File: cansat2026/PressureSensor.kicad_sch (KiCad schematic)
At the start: 2 parts, among them U601 AE-BME280

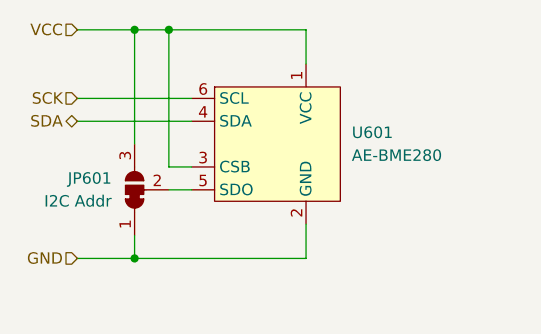
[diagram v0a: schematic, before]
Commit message: Update: いろいろした
無線変えた
カメラのコネクタ変えた
i2cセンサ変えた
電源変えた:1.2V,3.8V,3.3V
IOエキスパンダ追加
FPGA追加
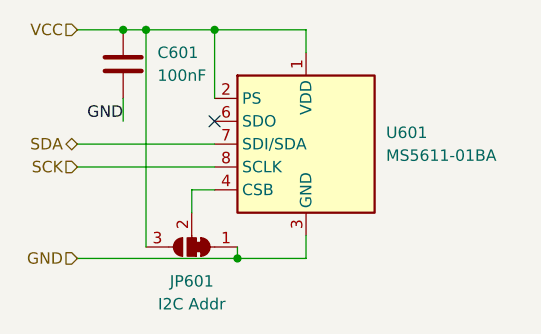
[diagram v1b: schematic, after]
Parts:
- removed U601: AE-BME280, Project:AE-BME280, symbol Project:AE-BME280
- added C601: 100nF, Capacitor_SMD:C_0402_1005Metric, symbol Device:C
- added U601: MS5611-01BA, Package_LGA:LGA-8_3x5mm_P1.25mm, symbol Sensor_Pressure:MS5611-01BA
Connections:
- net GND: now also C601.2, U601.3 (GND)
- net SCK: now also U601.8 (SCLK)
- net SDA: now also U601.7 (SDI/SDA)
- net VCC: now also C601.1, U601.1 (VDD), U601.2 (PS)
- net at JP601.2 (C): now also U601.4 (CSB), U601.5 (CSB)
- no-connect marks 0 -> 1
